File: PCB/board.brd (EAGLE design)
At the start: 30 x 30 mm, 38 parts, among them IC1 W25Q32JVSSIQ, J1 USB-TYPE-C-31-M-12, Q1 S8050, Q2 S8050, U1 AMS1117_SOT223, U2 CH340C, U3 ESP8266EX, X1 SMA, Y1 40Mhz

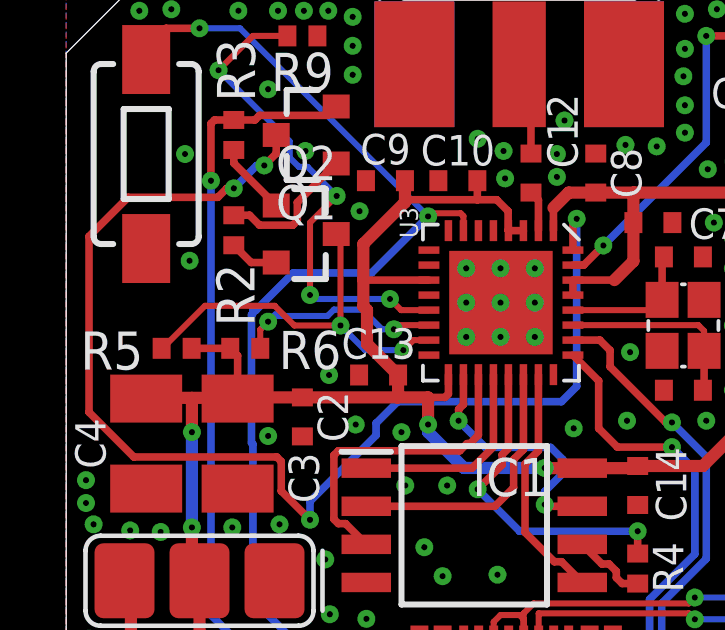
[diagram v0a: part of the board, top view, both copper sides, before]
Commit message: library update
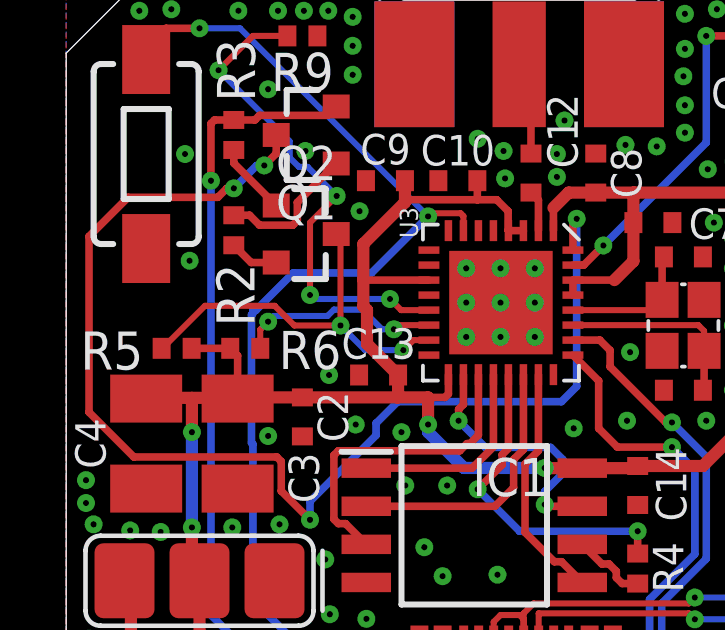
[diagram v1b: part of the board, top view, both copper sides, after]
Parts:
- U3: device angrypig7-IC:ESP8266EX -> angrypig7-IC-MCU:ESP8266EX
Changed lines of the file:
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@@
 <setting verticaltext="up"/>
 </settings>
-<grid distance="5" unitdist="mil" unit="mil" style="lines" multiple="1" display="yes" altdistance="5" altunitdist="mil" altunit="mil"/>
+<grid distance="10" unitdist="mil" unit="mil" style="lines" multiple="1" display="yes" altdistance="5" altunitdist="mil" altunit="mil"/>
 <layers>
 <layer number="1" name="Top" color="4" fill="1" visible="yes" active="yes"/>
@@
 <attribute name="SPICEPREFIX" value="C" x="41.783" y="39.243" size="1.778" layer="27" rot="R90" display="off"/>
 </element>
-<element name="U3" library="angrypig7-IC" package="ESP8266EX" value="ESP8266EX" x="14.492" y="19.685" smashed="yes" rot="R270">
+<element name="U3" library="angrypig7-IC-MCU" package="ESP8266EX" value="ESP8266EX" x="14.492" y="19.685" smashed="yes" rot="R270">
 <attribute name="LCSC" value="C77967" x="14.492" y="19.685" size="1.778" layer="27" rot="R270" display="off"/>
 <attribute name="NAME" x="11.423" y="22.352" size="0.6096" layer="21" font="vector" ratio="15" rot="R270" align="center"/>
@@
 <contactref element="R6" pad="1"/>
 <via x="10.922" y="18.796" extent="1-16" drill="0.2"/>
-<wire x1="6.985" y1="19.304" x2="6.9215" y2="19.2405" width="0.2032" layer="16"/>
 <via x="6.731" y="19.05" extent="1-16" drill="0.2"/>
 <wire x1="6.9215" y1="19.2405" x2="6.731" y2="19.05" width="0.2032" layer="16"/>
